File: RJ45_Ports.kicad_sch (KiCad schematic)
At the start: 17 parts, among them J2 R-RJ45R10P-B000, J3 R-RJ45R10P-B000

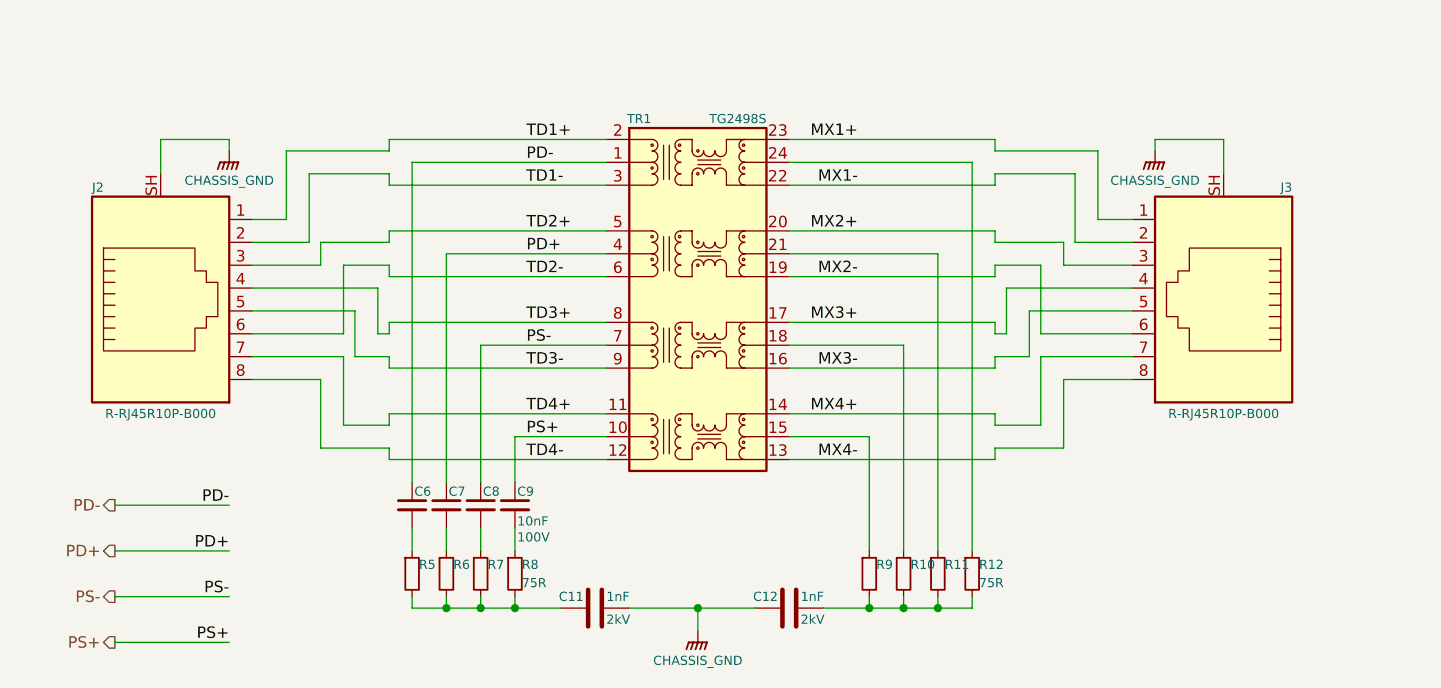
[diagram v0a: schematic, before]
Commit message: 1
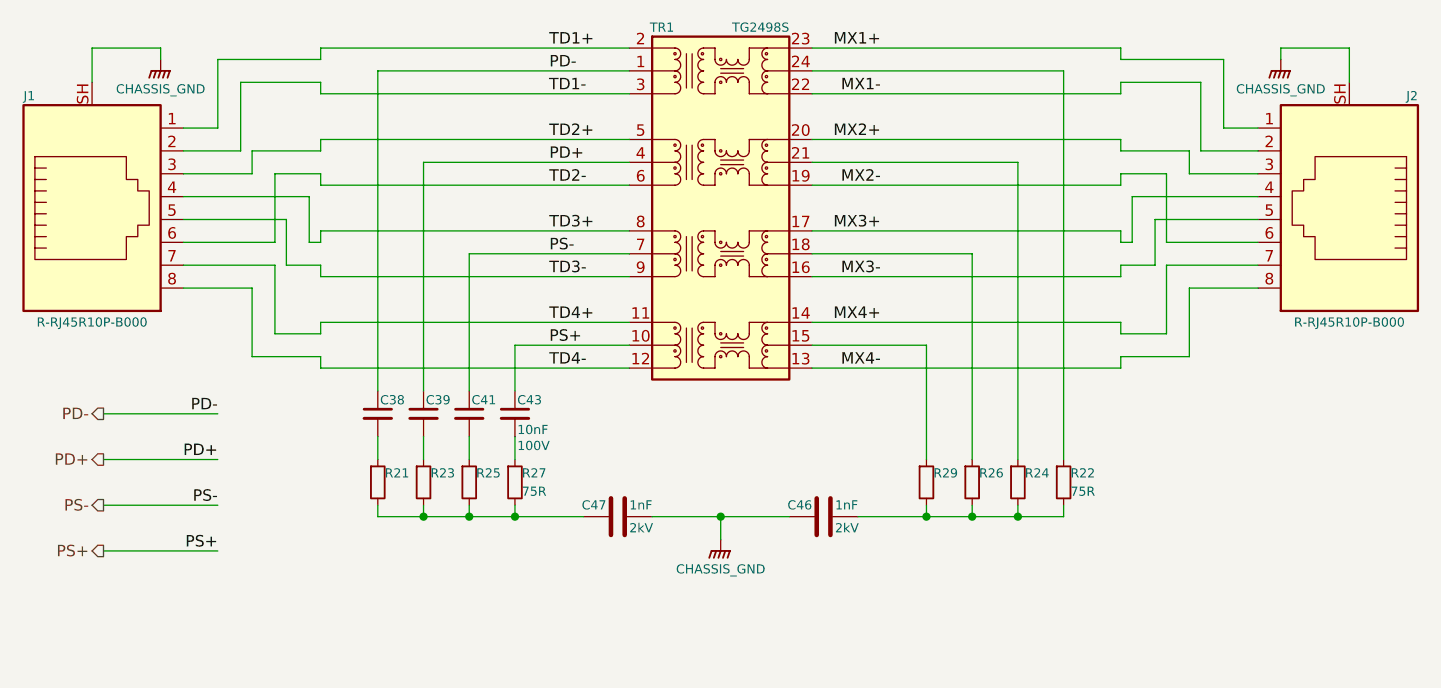
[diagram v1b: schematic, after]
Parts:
- renumbered C6 to C38, C7 to C39, C8 to C41, C9 to C43, C12 to C46, C11 to C47, J2 to J1, J3 to J2, R5 to R21, R12 to R22, R6 to R23, R11 to R24, R7 to R25, R10 to R26, R8 to R27, R9 to R29
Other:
- moved on the sheet: C38, C39, C41, C43, C46, C47, J1, J2, R21, R22, R23, R24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

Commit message: add ci
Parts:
- TR1: symbol Transformer:PT61020EL -> PoE_Splitter:TG2498S
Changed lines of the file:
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@@
 	)
 	(symbol
-		(lib_id "Transformer:PT61020EL")
+		(lib_id "PoE_Splitter:TG2498S")
 		(at 146.05 76.2 0)
 		(unit 1)
@@
 			(effects
 				(font
-					(size 1.016 1.016)
+					(size 1.27 1.27)
 				)
 			)
 		)
-		(property "Datasheet" "https://www.bourns.com/pdfs/PT61020.pdf"
+		(property "Datasheet" "https://www.lcsc.com/datasheet/C37328808.pdf"
 			(at 146.05 76.2 0)
 			(hide yes)
@@
 			(effects
 				(font
-					(size 1.016 1.016)
+					(size 1.27 1.27)
 				)
 			)
 		)
-		(property "Description" "10/100/1000 Base-T Ethernet Transformer, SMD-24"
+		(property "Description" "10GBASE-T POE+ Transformer Module, TG2498S"
 			(at 146.05 76.2 0)
 			(hide yes)
@@
 			(effects
 				(font
-					(size 1.016 1.016)
+					(size 1.27 1.27)
 				)
 			)
